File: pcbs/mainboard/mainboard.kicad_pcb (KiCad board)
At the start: 4 copper layers, 49 parts, among them J1 USB_B_Micro, J10 STAT_LED, J11 nReset_Button, J12 VBUS, J2 key_row_0, J3 key_row_1, J4 key_row_2, J5 ICSP, J6 JTAG, J7 Crank, J8 GPIO, J9 I2C, SW1 nReset, SW2 HWB, U1 ATmega32U4-AU, U2 USBLC6-2SC6, U3 XC6206P332MR, U4 XC9572XL-10VQG44C, Y1 16MHz

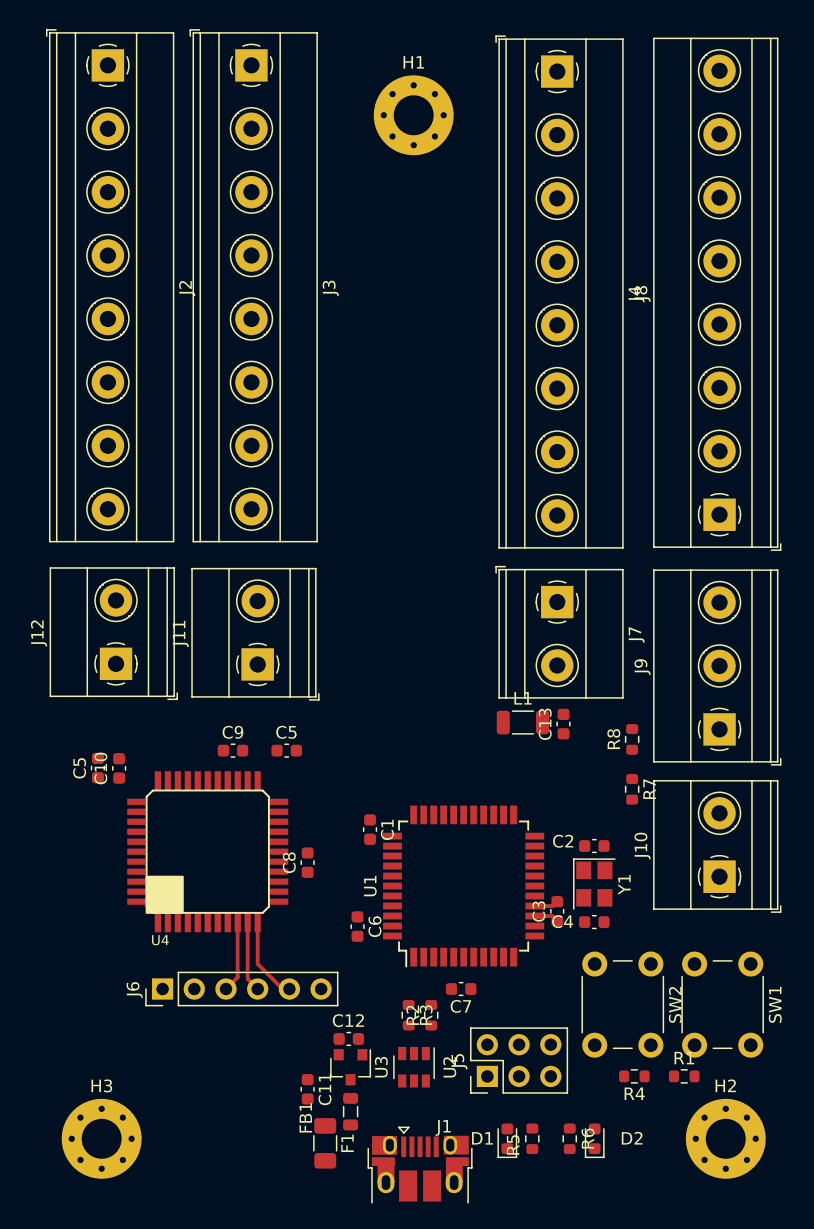
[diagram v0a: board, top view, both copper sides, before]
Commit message: Add first draft of mainboard routing
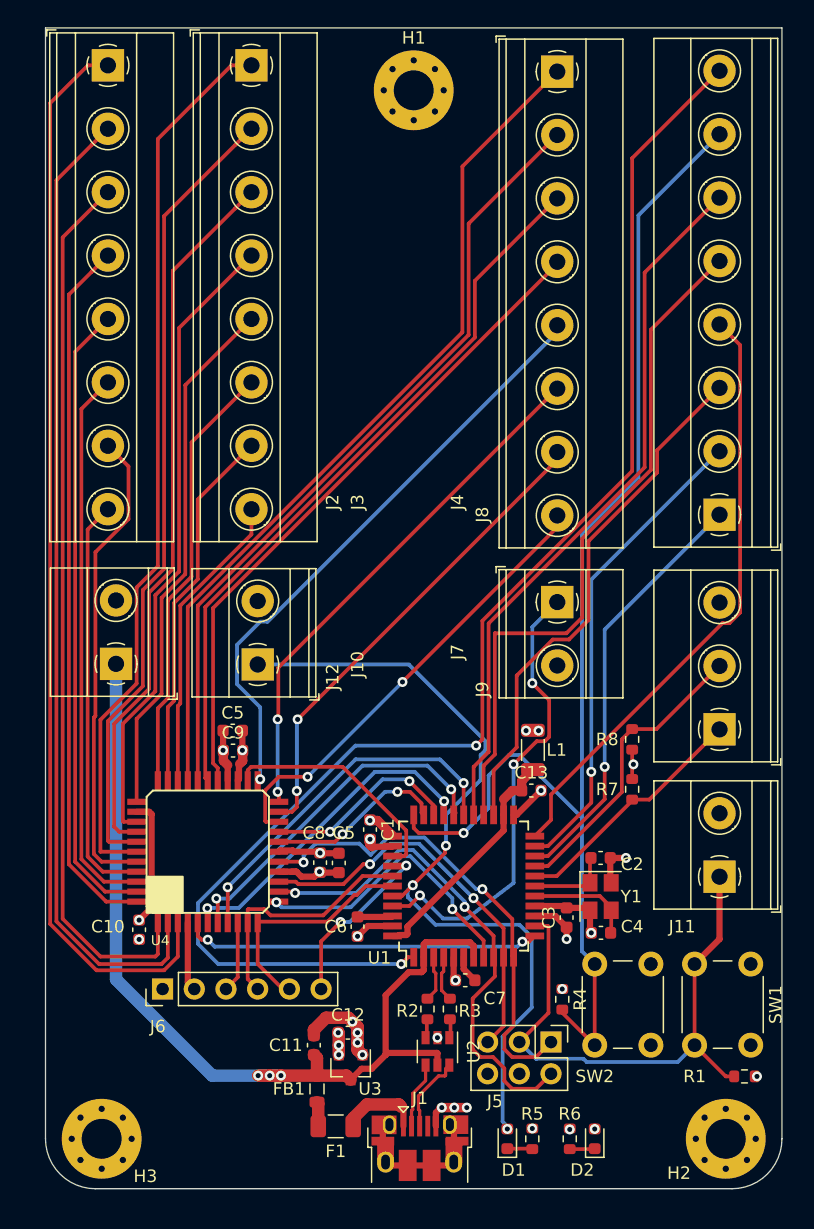
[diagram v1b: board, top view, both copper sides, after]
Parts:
- moved J10 40.7 mm to (116.0, 80.0)
- moved J11 40.7 mm to (153.0, 97.0)
- moved C5 20.7 mm to (122.5, 95.9)
- moved C10 13.0 mm to (106.5, 101.2), turned to 270 degrees
- moved R4 8.45 mm to (140.4, 106.8), turned to 270 degrees
- moved C13 5.91 mm to (137.9, 90.1), turned to 0 degrees
- moved J5 5.79 mm to (139.5, 110.2), turned to 270 degrees
- moved R1 4.82 mm to (155.0, 113.0), turned to 180 degrees
- moved C5 4.61 mm to (114.0, 85.3)
- moved C11 3.57 mm to (120.5, 110.5), turned to 90 degrees
- moved FB1 3.25 mm to (120.8, 114.0)
- moved L1 2.34 mm to (138.1, 86.8), turned to 270 degrees
- moved U2 2.26 mm to (130.4, 111.0)
- moved H1 2.00 mm to (128.5, 34.0)
- moved J1 1.65 mm to (129.0, 118.8)
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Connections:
- net Net-(R2-Pad2) renamed /D+
- net Net-(R3-Pad1) renamed /D-
- U4 pad 12: MISO -> /key_bus0
- U4 pad 13: MOSI -> SCK
- U4 pad 14: SCK -> MOSI
- U4 pad 16: /key_bus0 -> MISO
- U4 pad 18: /key_sel0 -> /key_sel1
- U4 pad 19: /key_sel1 -> /key_sel0
- U4 pad 40: key_row0_7 -> key_row0_6
- U4 pad 41: key_row0_6 -> key_row0_7
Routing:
- net GPIO7: track 0.00 -> 111.1 mm, vias 0 -> 2
- net GPIO6_HWB: track 0.00 -> 102.8 mm, vias 0 -> 1
- net key_row0_0: track 0.00 -> 86.6 mm
- net key_row0_1: track 0.00 -> 78.6 mm
- net VBUS: track 0.00 -> 75.6 mm, vias 0 -> 3
- net key_row1_0: track 0.00 -> 71.8 mm
- net key_row0_2: track 0.00 -> 71.2 mm
- net key_row2_0: track 0.00 -> 69.1 mm
- net STAT_LED: track 0.00 -> 65.6 mm, vias 0 -> 3
- net key_row1_1: track 0.00 -> 64.1 mm
- net key_row2_1: track 0.00 -> 63.6 mm
- net key_row2_2: track 0.00 -> 58.4 mm
- net GPIO5: track 0.00 -> 57.6 mm
- net key_row1_2: track 0.00 -> 57.4 mm
- net key_row0_3: track 0.00 -> 56.7 mm
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- added copper zone on In2.Cu, net +3V3
- added copper zone on In1.Cu, net GND
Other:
- board outline added: 59 x 93 mm
